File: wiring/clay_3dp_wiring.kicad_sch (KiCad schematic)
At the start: 1 part, among them J2 R3.CS

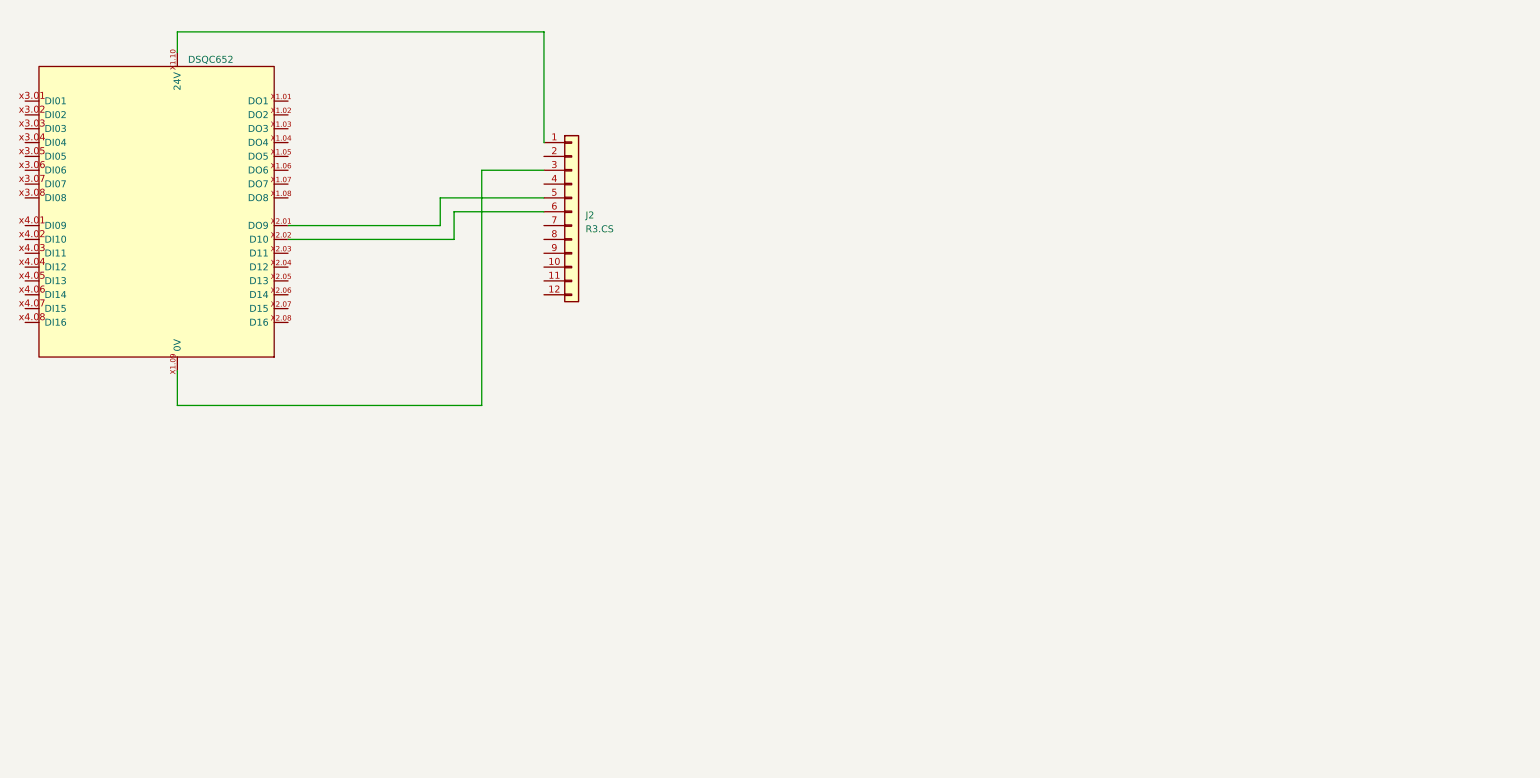
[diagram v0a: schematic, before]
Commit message: update, but need to check references on hierchial sheets
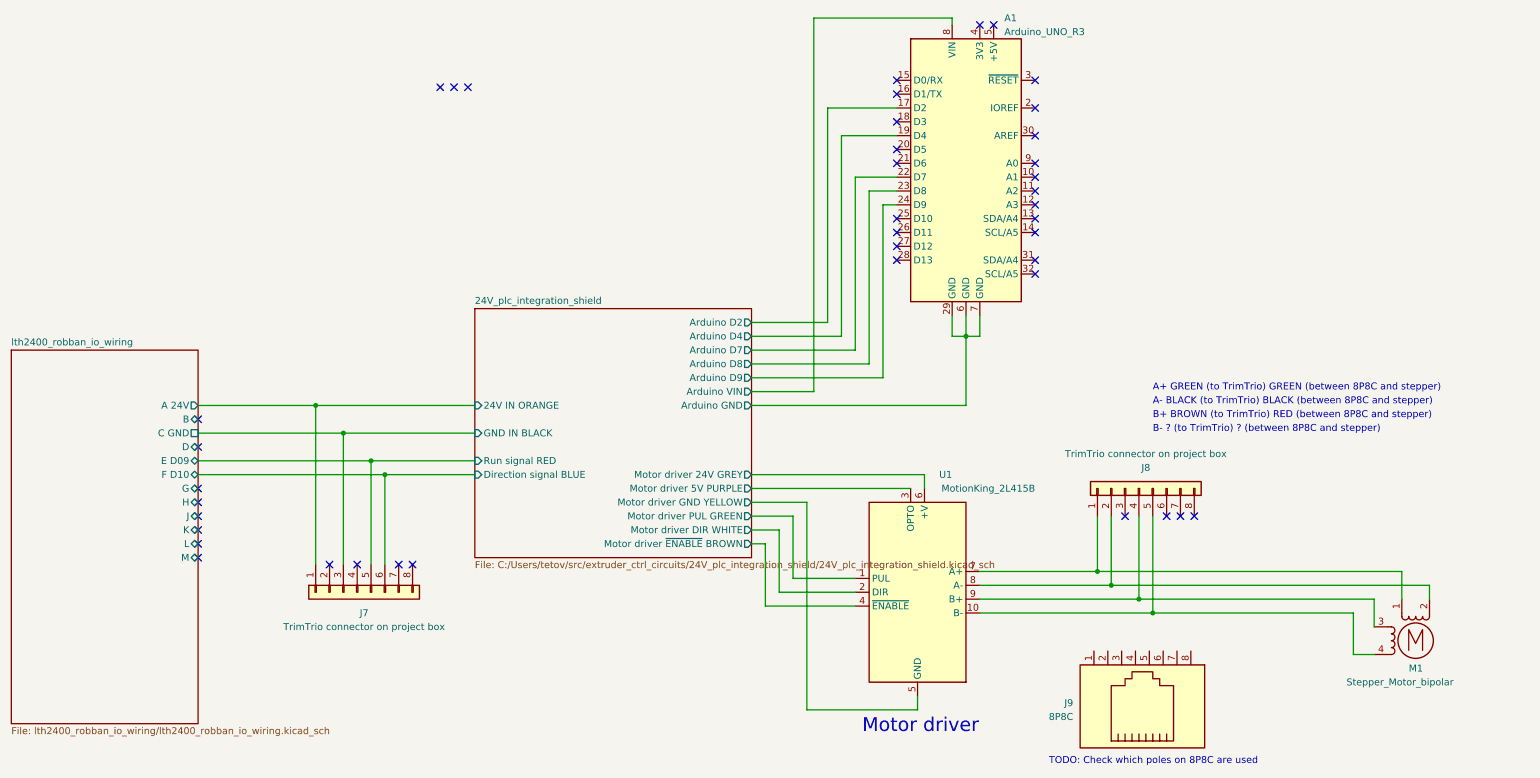
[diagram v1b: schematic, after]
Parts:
- removed J2: R3.CS, symbol Connector_Generic:Conn_01x12
- added A1: Arduino_UNO_R3, Module:Arduino_UNO_R3, symbol MCU_Module:Arduino_UNO_R3
- added J7, J8: TrimTrio connector on project box, symbol Connector_Generic:Conn_01x08
- added J9: 8P8C, symbol Connector:8P8C
- added M1: Stepper_Motor_bipolar, symbol Motor:Stepper_Motor_bipolar
- added U1: MotionKing_2L415B, symbol clay_3dp_wiring:MotionKing_2L415B
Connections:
- new net: J8.1 (Pin_1), M1.1, U1.7 (A+)
- new net: J8.2 (Pin_2), M1.2 (-), U1.8 (A-)
- new net: J8.4 (Pin_4), M1.3, U1.9 (B+)
- new net: J8.5 (Pin_5), M1.4, U1.10 (B-)
- new net 24V_plc_integration_shield/24V IN ORANGE: J7.1 (Pin_1)
- new net 24V_plc_integration_shield/Arduino D2: A1.17 (D2)
- new net 24V_plc_integration_shield/Arduino D4: A1.19 (D4)
- new net 24V_plc_integration_shield/Arduino D7: A1.22 (D7)
- new net 24V_plc_integration_shield/Arduino D8: A1.23 (D8)
- new net 24V_plc_integration_shield/Arduino D9: A1.24 (D9)
- new net 24V_plc_integration_shield/Arduino GND: A1.29 (GND), A1.6 (GND), A1.7 (GND)
- new net 24V_plc_integration_shield/Arduino VIN: A1.8 (VIN)
- new net 24V_plc_integration_shield/Direction signal BLUE: J7.6 (Pin_6)
- new net 24V_plc_integration_shield/GND IN BLACK: J7.3 (Pin_3)
- new net 24V_plc_integration_shield/Motor driver 24V GREY: U1.6 (+V)
- new net 24V_plc_integration_shield/Motor driver 5V PURPLE: U1.3 (OPTO)
- new net 24V_plc_integration_shield/Motor driver DIR WHITE: U1.2 (DIR)
- new net 24V_plc_integration_shield/Motor driver GND YELLOW: U1.5 (GND)
- new net 24V_plc_integration_shield/Motor driver PUL GREEN: U1.1 (PUL)
- new net 24V_plc_integration_shield/Motor driver ~{ENABLE} BROWN: U1.4 (~{ENABLE})
- new net 24V_plc_integration_shield/Run signal RED: J7.5 (Pin_5)
- no-connect marks 0 -> 41
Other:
- added sheet 24V_plc_integration_shield (C:/Users/tetov/src/extruder_ctrl_circuits/24V_plc_integration_shield/24V_plc_integration_shield.kicad_sch)
- added sheet lth2400_robban_io_wiring (lth2400_robban_io_wiring/lth2400_robban_io_wiring.kicad_sch)
- note added: "A+ GREEN (to TrimTrio) GREEN (between 8P8C and stepper)"
- note added: "A- BLACK (to TrimTrio) BLACK (between 8P8C and stepper)"
- note added: "B+ BROWN (to TrimTrio) RED (between 8P8C and stepper)"
- note added: "B- ? (to TrimTrio) ? (between 8P8C and stepper)"
- note added: "Motor driver"
- note added: "TODO: Check which poles on 8P8C are used"
